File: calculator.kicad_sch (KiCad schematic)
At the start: 40 parts, among them J1 Conn_01x04_Pin, J2 Conn_01x20_Socket, SW1 SW_Push, SW10 SW_Push, SW2 SW_Push, SW3 SW_Push, SW4 SW_Push, SW5 SW_Push, SW6 SW_Push, SW7 SW_Push, SW8 SW_Push, SW9 SW_Push, U1 STM32F103RETx, U2 AMS1117, Y1 Crystal

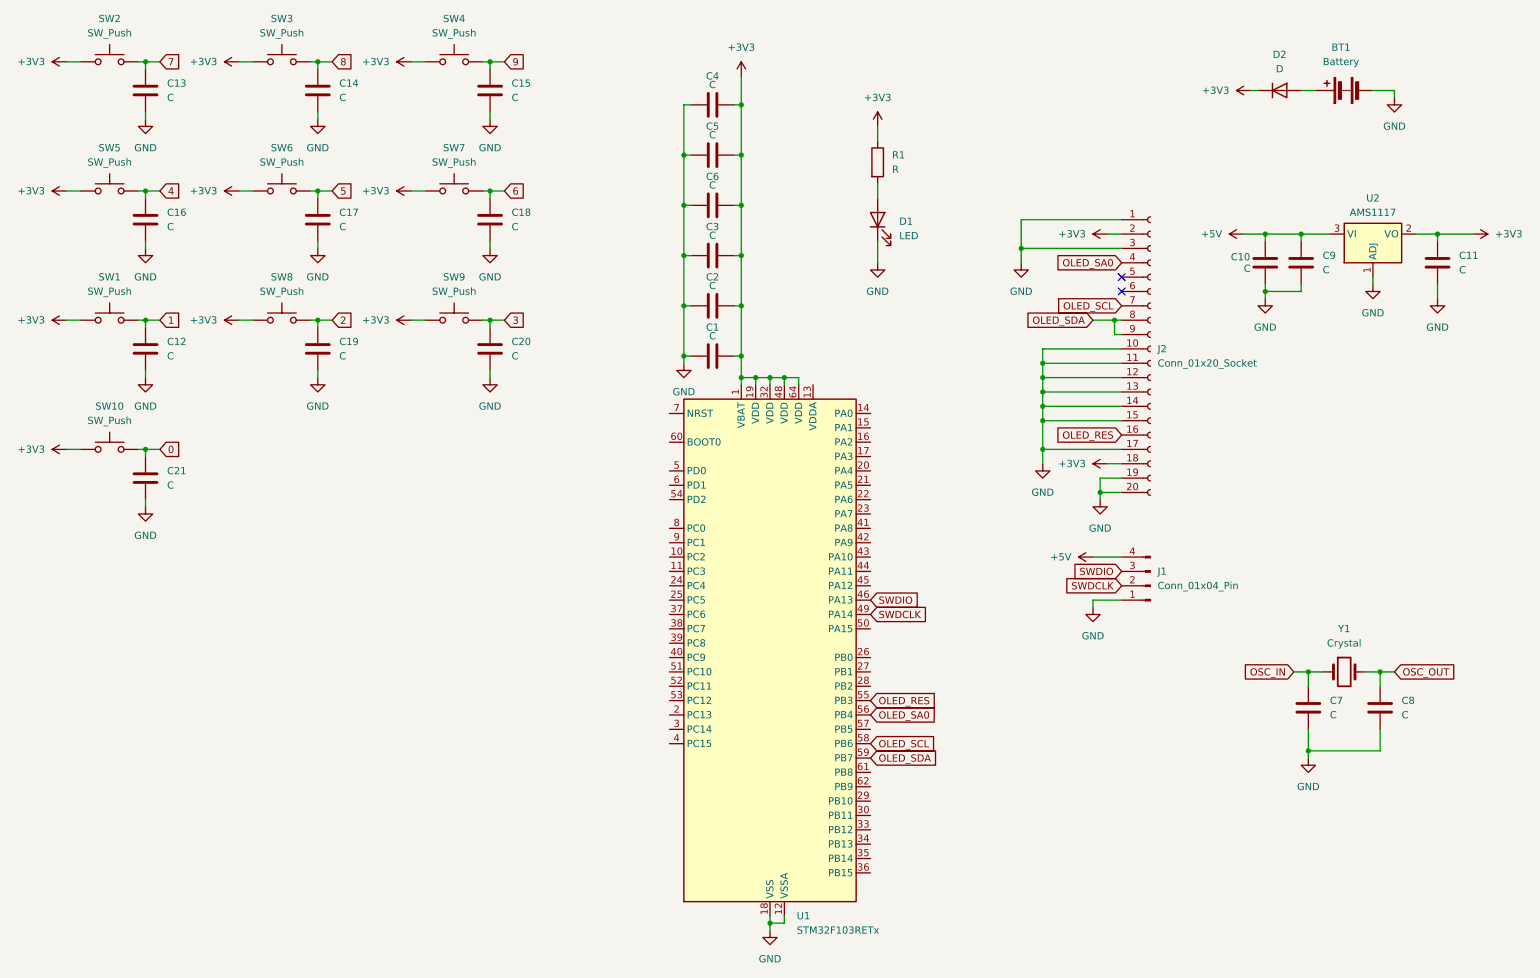
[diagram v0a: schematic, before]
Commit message: Design more of the pcb
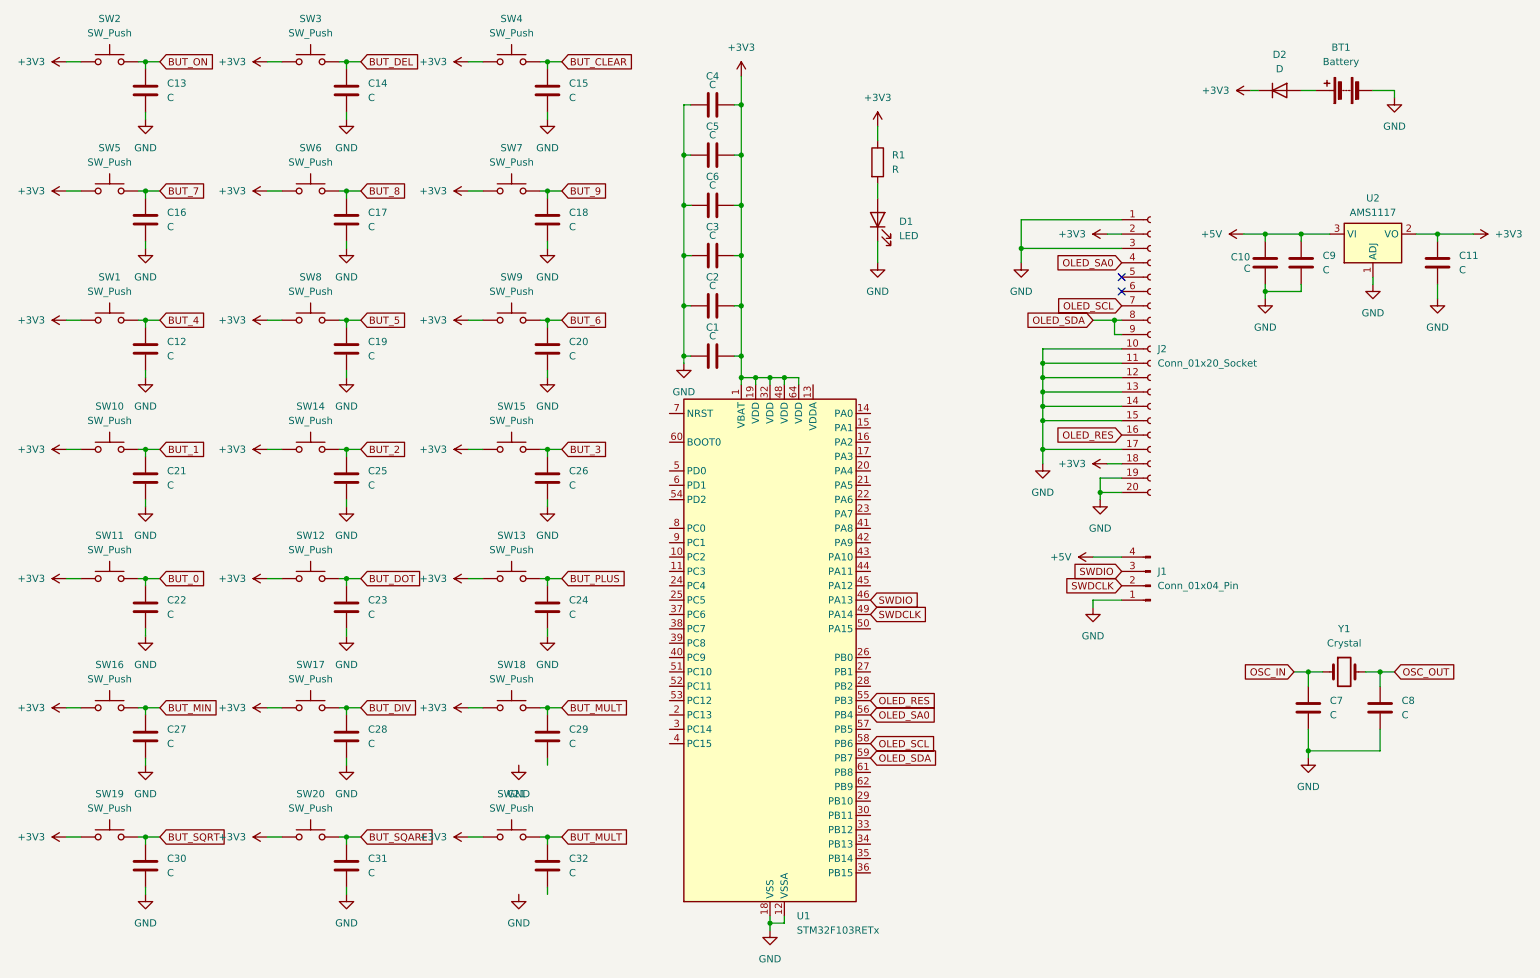
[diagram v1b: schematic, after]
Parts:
- added C22, C23, C24, C25, C26, C27, C28, C29, C30, C31, C32: C, symbol Device:C
- added SW11, SW12, SW13, SW14, SW15, SW16, SW17, SW18, SW19, SW20, SW21: SW_Push, symbol Switch:SW_Push
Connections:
- net +3V3: now also SW11.1, SW12.1, SW13.1, SW14.1, SW15.1, SW16.1, SW17.1, SW18.1, SW19.1, SW20.1, SW21.1
- net GND: now also C22.2, C23.2, C24.2, C25.2, C26.2, C27.2, C28.2, C30.2, C31.2
- net 0 renamed BUT_1
- net 1 renamed BUT_4
- net 2 renamed BUT_5
- net 3 renamed BUT_6
- net 4 renamed BUT_7
- net 5 renamed BUT_8
- net 6 renamed BUT_9
- net 7 renamed BUT_ON
- net 8 renamed BUT_DEL
- net 9 renamed BUT_CLEAR
- new net BUT_0: C22.1, SW11.2
- new net BUT_2: C25.1, SW14.2
- new net BUT_3: C26.1, SW15.2
- new net BUT_DIV: C28.1, SW17.2
- new net BUT_DOT: C23.1, SW12.2
- new net BUT_MIN: C27.1, SW16.2
- new net BUT_MULT: C29.1, C32.1, SW18.2, SW21.2
- new net BUT_PLUS: C24.1, SW13.2
- new net BUT_SQARE: C31.1, SW20.2
- new net BUT_SQRT: C30.1, SW19.2
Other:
- moved on the sheet: C14, C15, C17, C18, C19, C20, SW3, SW4, SW6, SW7, SW8, SW9
